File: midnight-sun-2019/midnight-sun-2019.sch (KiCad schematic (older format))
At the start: 70 parts, among them J101 Conn_01x02, J102 Conn_01x02, J103 USB_B_Micro, SW101 SW_SPDT, SW102 SW_SPDT, SW103 SW_SPDT, U101 74HC14, U102 74HC595, U103 74HC595, U104 74HC595, U105 74HC86, U106 74HC86, U107 74HC86, U108 74HC86, U109 74HC14, U110 74HC14, U111 74HC86, U112 74HC86, U113 74HC86, U114 74HC86, U115 74HC14, U116 74HC14

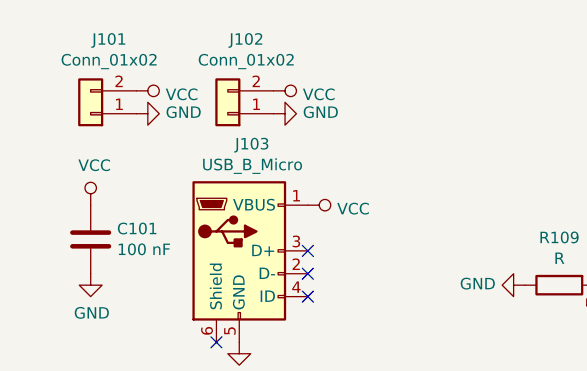
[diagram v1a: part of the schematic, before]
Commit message: Finish wiring everything up
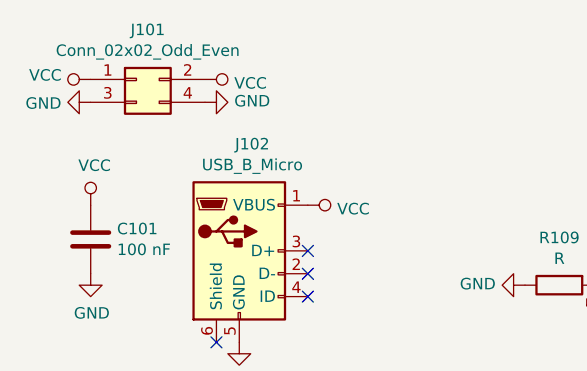
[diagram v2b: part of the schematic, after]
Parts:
- removed J101: Conn_01x02, Connector_PinSocket_2.54mm:PinSocket_1x02_P2.54mm_Vertical, symbol Connector_Generic:Conn_01x02
- removed J102: Conn_01x02, Connector_PinHeader_2.54mm:PinHeader_1x02_P2.54mm_Vertical, symbol Connector_Generic:Conn_01x02
- added J101: Conn_02x02_Odd_Even, Connector_PinHeader_2.54mm:PinHeader_2x02_P2.54mm_Vertical, symbol Connector_Generic:Conn_02x02_Odd_Even
- renumbered J103 to J102
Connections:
- net GND: now also J101.3 (Pin_3), J101.4 (Pin_4)
- net VCC: now also J101.1 (Pin_1), J101.2 (Pin_2)
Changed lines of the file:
@@
 Text Label 3250 2000 2    50   ~ 0
 rst
-$Comp
-L Connector_Generic:Conn_01x02 J101
-U 1 1 5CEEE3A8
-P 750 950
-F 0 "J101" H 668 625 50  0000 C CNN
-F 1 "Conn_01x02" H 668 716 50  0000 C CNN
-F 2 "Connector_PinSocket_2.54mm:PinSocket_1x02_P2.54mm_Vertical" H 750 950 50  0001 C CNN
-F 3 "~" H 750 950 50  0001 C CNN
-	1    750  950
-	-1   0    0    1
-$EndComp
 Text Label 4050 3900 0    50   ~ 0
 x0
@@
 NoConn ~ 4050 2200
 $Comp
-L power:GND #PWR0104
+L power:GND #PWR0114
 U 1 1 5CEEF634
-P 950 950
-F 0 "#PWR0104" H 950 700 50  0001 C CNN
-F 1 "GND" V 955 822 50  0000 R CNN
-F 2 "" H 950 950 50  0001 C CNN
-F 3 "" H 950 950 50  0001 C CNN
-	1    950  950
+P 1250 900
+F 0 "#PWR0114" H 1250 650 50  0001 C CNN
+F 1 "GND" V 1255 772 50  0000 R CNN
+F 2 "" H 1250 900 50  0001 C CNN
+F 3 "" H 1250 900 50  0001 C CNN
+	1    1250 900
 	0    -1   -1   0
 $EndComp
@@
 NoConn ~ 1700 1550
 $Comp
-L Connector:USB_B_Micro J103
+L Connector:USB_B_Micro J102
 U 1 1 76EFDB97
 P 1400 1550
-F 0 "J103" H 1457 2017 50  0000 C CNN
+F 0 "J102" H 1457 2017 50  0000 C CNN
 F 1 "USB_B_Micro" H 1457 1926 50  0000 C CNN
 F 2 "electrokit:USB_Micro-B_Electrokit_anr41011019" H 1550 1500 50  0001 C CNN
@@
 $EndComp
 $Comp
-L power:VCC #PWR0103
+L power:VCC #PWR0113
 U 1 1 76F38640
-P 950 850
-F 0 "#PWR0103" H 950 700 50  0001 C CNN
-F 1 "VCC" V 967 978 50  0000 L CNN
-F 2 "" H 950 850 50  0001 C CNN
-F 3 "" H 950 850 50  0001 C CNN
-	1    950  850
+P 1250 800
+F 0 "#PWR0113" H 1250 650 50  0001 C CNN
+F 1 "VCC" V 1267 928 50  0000 L CNN
+F 2 "" H 1250 800 50  0001 C CNN
+F 3 "" H 1250 800 50  0001 C CNN
+	1    1250 800
 	0    1    1    0
 $EndComp
@@
 $EndComp
 $Comp
-L power:GND #PWR0113
+L power:GND #PWR0115
 U 1 1 76FDF255
 P 1350 2600
-F 0 "#PWR0113" H 1350 2350 50  0001 C CNN
+F 0 "#PWR0115" H 1350 2350 50  0001 C CNN
 F 1 "GND" H 1355 2427 50  0000 C CNN
 F 2 "" H 1350 2600 50  0001 C CNN
@@
 $EndComp
 $Comp
-L power:GND #PWR0102
+L power:GND #PWR0104
 U 1 1 5CBF3918
 P 750 1650
-F 0 "#PWR0102" H 750 1400 50  0001 C CNN
+F 0 "#PWR0104" H 750 1400 50  0001 C CNN
 F 1 "GND" H 755 1477 50  0000 C CNN
 F 2 "" H 750 1650 50  0001 C CNN
@@
 $EndComp
 $Comp
-L power:VCC #PWR0101
+L power:VCC #PWR0103
 U 1 1 5CBE8005
 P 750 1350
-F 0 "#PWR0101" H 750 1200 50  0001 C CNN
+F 0 "#PWR0103" H 750 1200 50  0001 C CNN
 F 1 "VCC" H 767 1523 50  0000 C CNN
 F 2 "" H 750 1350 50  0001 C CNN
@@
 $EndComp
 $Comp
-L power:GND #PWR0114
+L power:GND #PWR0116
 U 1 1 5CC60BF0
 P 1400 1950
-F 0 "#PWR0114" H 1400 1700 50  0001 C CNN
+F 0 "#PWR0116" H 1400 1700 50  0001 C CNN
 F 1 "GND" H 1405 1777 50  0000 C CNN
 F 2 "" H 1400 1950 50  0001 C CNN
@@
 b15
 $Comp
-L Connector_Generic:Conn_01x02 J102
-U 1 1 5FC8D734
-P 1350 950
-F 0 "J102" H 1268 625 50  0000 C CNN
-F 1 "Conn_01x02" H 1268 716 50  0000 C CNN
-F 2 "Connector_PinHeader_2.54mm:PinHeader_1x02_P2.54mm_Vertical" H 1350 950 50  0001 C CNN
-F 3 "~" H 1350 950 50  0001 C CNN
-	1    1350 950
-	-1   0    0    1
-$EndComp
-$Comp
-L power:GND #PWR0116
-U 1 1 5FC8D73A
-P 1550 950
-F 0 "#PWR0116" H 1550 700 50  0001 C CNN
-F 1 "GND" V 1555 822 50  0000 R CNN
-F 2 "" H 1550 950 50  0001 C CNN
-F 3 "" H 1550 950 50  0001 C CNN
-	1    1550 950
+L Connector_Generic:Conn_02x02_Odd_Even J101
+U 1 1 5F1504BD
+P 950 800
+F 0 "J101" H 1000 1017 50  0000 C CNN
+F 1 "Conn_02x02_Odd_Even" H 1000 926 50  0000 C CNN
+F 2 "Connector_PinHeader_2.54mm:PinHeader_2x02_P2.54mm_Vertical" H 950 800 50  0001 C CNN
+F 3 "~" H 950 800 50  0001 C CNN
+	1    950  800
+	1    0    0    -1
+$EndComp
+$Comp
+L power:GND #PWR0102
+U 1 1 5F16ECDF
+P 750 900
+F 0 "#PWR0102" H 750 650 50  0001 C CNN
+F 1 "GND" V 755 772 50  0000 R CNN
+F 2 "" H 750 900 50  0001 C CNN
+F 3 "" H 750 900 50  0001 C CNN
+	1    750  900
+	0    1    1    0
+$EndComp
+$Comp
+L power:VCC #PWR0101
+U 1 1 5F171491
+P 750 800
+F 0 "#PWR0101" H 750 650 50  0001 C CNN
+F 1 "VCC" V 768 927 50  0000 L CNN
+F 2 "" H 750 800 50  0001 C CNN
+F 3 "" H 750 800 50  0001 C CNN
+	1    750  800
 	0    -1   -1   0
 $EndComp
-$Comp
-L power:VCC #PWR0115
-U 1 1 5FC8D740
-P 1550 850
-F 0 "#PWR0115" H 1550 700 50  0001 C CNN
-F 1 "VCC" V 1567 978 50  0000 L CNN
-F 2 "" H 1550 850 50  0001 C CNN
-F 3 "" H 1550 850 50  0001 C CNN
-	1    1550 850
-	0    1    1    0
-$EndComp
-Wire Wire Line
+Wire Wire Line

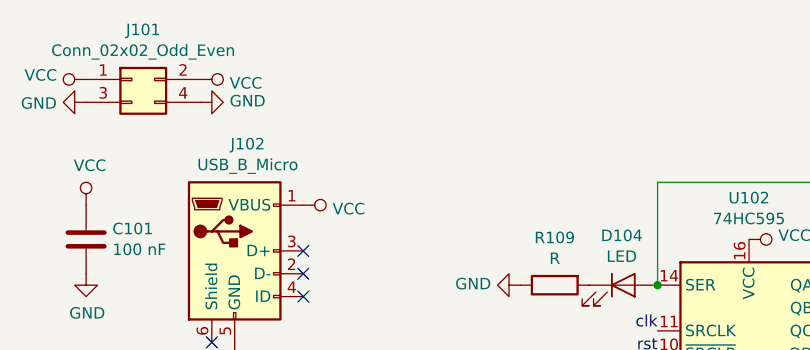
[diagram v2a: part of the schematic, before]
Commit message: Add battery holders
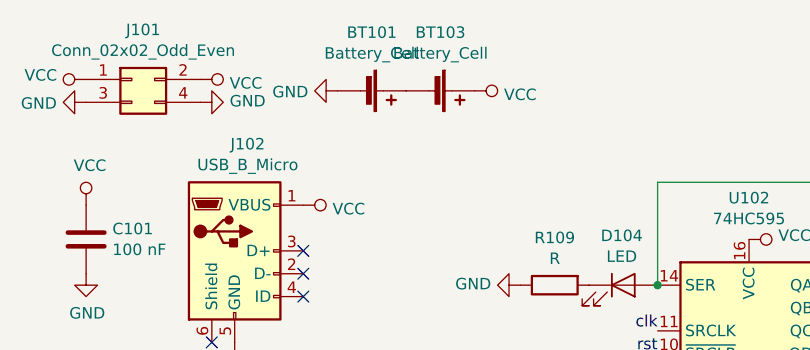
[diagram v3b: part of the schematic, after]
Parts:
- added BT101, BT103: Battery_Cell, electrokit:BatteryHolder_CR2016_CR2025_CR2032_22mm, symbol Device:Battery_Cell
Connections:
- net GND: now also BT101.2 (-)
- net VCC: now also BT103.1 (+)
- new net: BT101.1 (+), BT103.2 (-)
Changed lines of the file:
@@
 $EndComp
 $Comp
-L power:GND #PWR0124
+L power:GND #PWR0126
 U 1 1 5CC0CF82
 P 3250 2300
-F 0 "#PWR0124" H 3250 2050 50  0001 C CNN
+F 0 "#PWR0126" H 3250 2050 50  0001 C CNN
 F 1 "GND" V 3255 2172 50  0000 R CNN
 F 2 "" H 3250 2300 50  0001 C CNN
@@
 clk
 $Comp
-L power:VCC #PWR0127
+L power:VCC #PWR0129
 U 1 1 5CC0F9A9
 P 3650 1500
-F 0 "#PWR0127" H 3650 1350 50  0001 C CNN
+F 0 "#PWR0129" H 3650 1350 50  0001 C CNN
 F 1 "VCC" V 3667 1628 50  0000 L CNN
 F 2 "" H 3650 1500 50  0001 C CNN
@@
 NoConn ~ 4050 2600
 $Comp
-L power:GND #PWR0126
+L power:GND #PWR0128
 U 1 1 5CC1B6EE
 P 3250 6150
-F 0 "#PWR0126" H 3250 5900 50  0001 C CNN
+F 0 "#PWR0128" H 3250 5900 50  0001 C CNN
 F 1 "GND" V 3255 6022 50  0000 R CNN
 F 2 "" H 3250 6150 50  0001 C CNN
@@
 clk
 $Comp
-L power:VCC #PWR0131
+L power:VCC #PWR0133
 U 1 1 5CC1B702
 P 3650 5350
-F 0 "#PWR0131" H 3650 5200 50  0001 C CNN
+F 0 "#PWR0133" H 3650 5200 50  0001 C CNN
 F 1 "VCC" V 3667 5478 50  0000 L CNN
 F 2 "" H 3650 5350 50  0001 C CNN
@@
 clk
 $Comp
-L power:GND #PWR0130
+L power:GND #PWR0132
 U 1 1 5CC1C9E9
 P 3650 5000
-F 0 "#PWR0130" H 3650 4750 50  0001 C CNN
+F 0 "#PWR0132" H 3650 4750 50  0001 C CNN
 F 1 "GND" V 3655 4872 50  0000 R CNN
 F 2 "" H 3650 5000 50  0001 C CNN
@@
 $EndComp
 $Comp
-L power:VCC #PWR0129
+L power:VCC #PWR0131
 U 1 1 5CC1C9EF
 P 3650 3700
-F 0 "#PWR0129" H 3650 3550 50  0001 C CNN
+F 0 "#PWR0131" H 3650 3550 50  0001 C CNN
 F 1 "VCC" V 3667 3828 50  0000 L CNN
 F 2 "" H 3650 3700 50  0001 C CNN
@@
 	3250 3450 3250 3900
 $Comp
-L power:GND #PWR0123
+L power:GND #PWR0124
 U 1 1 5CD027AA
 P 2650 1700
-F 0 "#PWR0123" H 2650 1450 50  0001 C CNN
+F 0 "#PWR0124" H 2650 1450 50  0001 C CNN
 F 1 "GND" V 2655 1572 50  0000 R CNN
 F 2 "" H 2650 1700 50  0001 C CNN
@@
 $EndComp
 $Comp
-L power:GND #PWR0133
+L power:GND #PWR0135
 U 1 1 5CD20D5E
 P 5450 4150
-F 0 "#PWR0133" H 5450 3900 50  0001 C CNN
+F 0 "#PWR0135" H 5450 3900 50  0001 C CNN
 F 1 "GND" V 5455 4022 50  0000 R CNN
 F 2 "" H 5450 4150 50  0001 C CNN
@@
 $EndComp
 $Comp
-L power:GND #PWR0134
+L power:GND #PWR0136
 U 1 1 5CD20D70
 P 5450 4550
-F 0 "#PWR0134" H 5450 4300 50  0001 C CNN
+F 0 "#PWR0136" H 5450 4300 50  0001 C CNN
 F 1 "GND" V 5455 4422 50  0000 R CNN
 F 2 "" H 5450 4550 50  0001 C CNN
@@
 $EndComp
 $Comp
-L power:GND #PWR0135
+L power:GND #PWR0137
 U 1 1 5CD20D82
 P 5450 4950
-F 0 "#PWR0135" H 5450 4700 50  0001 C CNN
+F 0 "#PWR0137" H 5450 4700 50  0001 C CNN
 F 1 "GND" V 5455 4822 50  0000 R CNN
 F 2 "" H 5450 4950 50  0001 C CNN
@@
 $EndComp
 $Comp
-L power:GND #PWR0136
+L power:GND #PWR0138
 U 1 1 5CD20D94
 P 5450 5350
-F 0 "#PWR0136" H 5450 5100 50  0001 C CNN
+F 0 "#PWR0138" H 5450 5100 50  0001 C CNN
 F 1 "GND" V 5455 5222 50  0000 R CNN
 F 2 "" H 5450 5350 50  0001 C CNN
@@
 $EndComp
 $Comp
-L power:GND #PWR0120
+L power:GND #PWR0121
 U 1 1 5DF27255
 P 2550 2600
-F 0 "#PWR0120" H 2550 2350 50  0001 C CNN
+F 0 "#PWR0121" H 2550 2350 50  0001 C CNN
 F 1 "GND" V 2555 2472 50  0000 R CNN
 F 2 "" H 2550 2600 50  0001 C CNN
@@
 $EndComp
 $Comp
-L power:GND #PWR0137
+L power:GND #PWR0139
 U 1 1 76A8EDEC
 P 5450 5750
-F 0 "#PWR0137" H 5450 5500 50  0001 C CNN
+F 0 "#PWR0139" H 5450 5500 50  0001 C CNN
 F 1 "GND" V 5455 5622 50  0000 R CNN
 F 2 "" H 5450 5750 50  0001 C CNN
@@
 $EndComp
 $Comp
-L power:GND #PWR0138
+L power:GND #PWR0140
 U 1 1 76A8EDF2
 P 5450 6150
-F 0 "#PWR0138" H 5450 5900 50  0001 C CNN
+F 0 "#PWR0140" H 5450 5900 50  0001 C CNN
 F 1 "GND" V 5455 6022 50  0000 R CNN
 F 2 "" H 5450 6150 50  0001 C CNN
@@
 $EndComp
 $Comp
-L power:GND #PWR0139
+L power:GND #PWR0141
 U 1 1 76A8EDF8
 P 5450 6550
-F 0 "#PWR0139" H 5450 6300 50  0001 C CNN
+F 0 "#PWR0141" H 5450 6300 50  0001 C CNN
 F 1 "GND" V 5455 6422 50  0000 R CNN
 F 2 "" H 5450 6550 50  0001 C CNN
@@
 $EndComp
 $Comp
-L power:GND #PWR0140
+L power:GND #PWR0142
 U 1 1 76A8EDFE
 P 5450 6950
-F 0 "#PWR0140" H 5450 6700 50  0001 C CNN
+F 0 "#PWR0142" H 5450 6700 50  0001 C CNN
 F 1 "GND" V 5455 6822 50  0000 R CNN
 F 2 "" H 5450 6950 50  0001 C CNN
@@
 $EndComp
 $Comp
-L power:GND #PWR0141
+L power:GND #PWR0143
 U 1 1 76B2DE98
 P 5450 7350
-F 0 "#PWR0141" H 5450 7100 50  0001 C CNN
+F 0 "#PWR0143" H 5450 7100 50  0001 C CNN
 F 1 "GND" V 5455 7222 50  0000 R CNN
 F 2 "" H 5450 7350 50  0001 C CNN
@@
 $EndComp
 $Comp
-L power:GND #PWR0142
+L power:GND #PWR0144
 U 1 1 76B2DE9E
 P 5450 7750
-F 0 "#PWR0142" H 5450 7500 50  0001 C CNN
+F 0 "#PWR0144" H 5450 7500 50  0001 C CNN
 F 1 "GND" V 5455 7622 50  0000 R CNN
 F 2 "" H 5450 7750 50  0001 C CNN
@@
 $EndComp
 $Comp
-L power:GND #PWR0143
+L power:GND #PWR0145
 U 1 1 76B2DEA4
 P 5450 8150
-F 0 "#PWR0143" H 5450 7900 50  0001 C CNN
+F 0 "#PWR0145" H 5450 7900 50  0001 C CNN
 F 1 "GND" V 5455 8022 50  0000 R CNN
 F 2 "" H 5450 8150 50  0001 C CNN
@@
 $EndComp
 $Comp
-L power:GND #PWR0144
+L power:GND #PWR0146
 U 1 1 76B2DEAA
 P 5450 8550
-F 0 "#PWR0144" H 5450 8300 50  0001 C CNN
+F 0 "#PWR0146" H 5450 8300 50  0001 C CNN
 F 1 "GND" V 5455 8422 50  0000 R CNN
 F 2 "" H 5450 8550 50  0001 C CNN
@@
 $EndComp
 $Comp
-L power:GND #PWR0145
+L power:GND #PWR0147
 U 1 1 76B2DEE0
 P 5450 8950
-F 0 "#PWR0145" H 5450 8700 50  0001 C CNN
+F 0 "#PWR0147" H 5450 8700 50  0001 C CNN
 F 1 "GND" V 5455 8822 50  0000 R CNN
 F 2 "" H 5450 8950 50  0001 C CNN
@@
 $EndComp
 $Comp
-L power:GND #PWR0146
+L power:GND #PWR0148
 U 1 1 76B2DEE6
 P 5450 9350
-F 0 "#PWR0146" H 5450 9100 50  0001 C CNN
+F 0 "#PWR0148" H 5450 9100 50  0001 C CNN
 F 1 "GND" V 5455 9222 50  0000 R CNN
 F 2 "" H 5450 9350 50  0001 C CNN
@@
 $EndComp
 $Comp
-L power:GND #PWR0147
+L power:GND #PWR0149
 U 1 1 76B2DEEC
 P 5450 9750
-F 0 "#PWR0147" H 5450 9500 50  0001 C CNN
+F 0 "#PWR0149" H 5450 9500 50  0001 C CNN
 F 1 "GND" V 5455 9622 50  0000 R CNN
 F 2 "" H 5450 9750 50  0001 C CNN
@@
 $EndComp
 $Comp
-L power:GND #PWR0148
+L power:GND #PWR0150
 U 1 1 76B2DEF2
 P 5450 10150
-F 0 "#PWR0148" H 5450 9900 50  0001 C CNN
+F 0 "#PWR0150" H 5450 9900 50  0001 C CNN
 F 1 "GND" V 5455 10022 50  0000 R CNN
 F 2 "" H 5450 10150 50  0001 C CNN
@@
 $EndComp
 $Comp
-L power:GND #PWR0132
+L power:GND #PWR0134
 U 1 1 5CC95636
 P 3650 6650
-F 0 "#PWR0132" H 3650 6400 50  0001 C CNN
+F 0 "#PWR0134" H 3650 6400 50  0001 C CNN
 F 1 "GND" H 3655 6477 50  0000 C CNN
 F 2 "" H 3650 6650 50  0001 C CNN
@@
 Connection ~ 3250 1700
 $Comp
-L power:GND #PWR0128
+L power:GND #PWR0130
 U 1 1 5CCDCBB3
 P 3650 2800
-F 0 "#PWR0128" H 3650 2550 50  0001 C CNN
+F 0 "#PWR0130" H 3650 2550 50  0001 C CNN
 F 1 "GND" H 3655 2627 50  0000 C CNN
 F 2 "" H 3650 2800 50  0001 C CNN
@@
 $EndComp
 $Comp
-L power:GND #PWR0125
+L power:GND #PWR0127
 U 1 1 5CCE0EF9
 P 3250 4500
-F 0 "#PWR0125" H 3250 4250 50  0001 C CNN
+F 0 "#PWR0127" H 3250 4250 50  0001 C CNN
 F 1 "GND" H 3255 4327 50  0000 C CNN
 F 2 "" H 3250 4500 50  0001 C CNN
@@
 $EndComp
 $Comp
-L power:GND #PWR0122
+L power:GND #PWR0123
 U 1 1 5CEC139D
 P 2550 5100
-F 0 "#PWR0122" H 2550 4850 50  0001 C CNN
+F 0 "#PWR0123" H 2550 4850 50  0001 C CNN
 F 1 "GND" V 2555 4972 50  0000 R CNN
 F 2 "" H 2550 5100 50  0001 C CNN
@@
 Connection ~ 1950 4100
 $Comp
-L power:GND #PWR0121
+L power:GND #PWR0122
 U 1 1 5CEBD2B8
 P 2550 3800
-F 0 "#PWR0121" H 2550 3550 50  0001 C CNN
+F 0 "#PWR0122" H 2550 3550 50  0001 C CNN
 F 1 "GND" V 2555 3672 50  0000 R CNN
 F 2 "" H 2550 3800 50  0001 C CNN
@@
 	0    -1   -1   0
 $EndComp
+$Comp
+L power:VCC #PWR0125
+U 1 1 5CF5D8FC
+P 2450 850
+F 0 "#PWR0125" H 2450 700 50  0001 C CNN
+F 1 "VCC" V 2467 978 50  0000 L CNN
+F 2 "" H 2450 850 50  0001 C CNN
+F 3 "" H 2450 850 50  0001 C CNN
+	1    2450 850
+	0    1    1    0
+$EndComp
+$Comp
+L power:GND #PWR0120
+U 1 1 5CF60359
+P 1850 850
+F 0 "#PWR0120" H 1850 600 50  0001 C CNN
+F 1 "GND" V 1855 722 50  0000 R CNN
+F 2 "" H 1850 850 50  0001 C CNN
+F 3 "" H 1850 850 50  0001 C CNN
+	1    1850 850
+	0    1    1    0
+$EndComp
+$Comp
+L Device:Battery_Cell BT101
+U 1 1 5CF621CA
+P 1950 850
+F 0 "BT101" V 1695 900 50  0000 C CNN
+F 1 "Battery_Cell" V 1786 900 50  0000 C CNN
+F 2 "electrokit:BatteryHolder_CR2016_CR2025_CR2032_22mm" V 1950 910 50  0001 C CNN
+F 3 "~" V 1950 910 50  0001 C CNN
+	1    1950 850
+	0    1    1    0
+$EndComp
+$Comp
+L Device:Battery_Cell BT103
+U 1 1 5CF653D3
+P 2250 850
+F 0 "BT103" V 1995 900 50  0000 C CNN
+F 1 "Battery_Cell" V 2086 900 50  0000 C CNN
+F 2 "electrokit:BatteryHolder_CR2016_CR2025_CR2032_22mm" V 2250 910 50  0001 C CNN
+F 3 "~" V 2250 910 50  0001 C CNN
+	1    2250 850
+	0    1    1    0
+$EndComp
 Wire Wire Line
 	6450 9800 7300 9800
@@
 	4300 3800 4300 6150
 Wire Bus Line
+	7050 6400 7050 11100
+Wire Bus Line
 	9800 2650 9800 5650
 Wire Bus Line
@@
 Wire Bus Line
 	4600 3800 4600 10050
-Wire Bus Line
-	7050 6400 7050 11100
 $EndSCHEMATC
